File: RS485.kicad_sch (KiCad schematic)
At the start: 0 parts

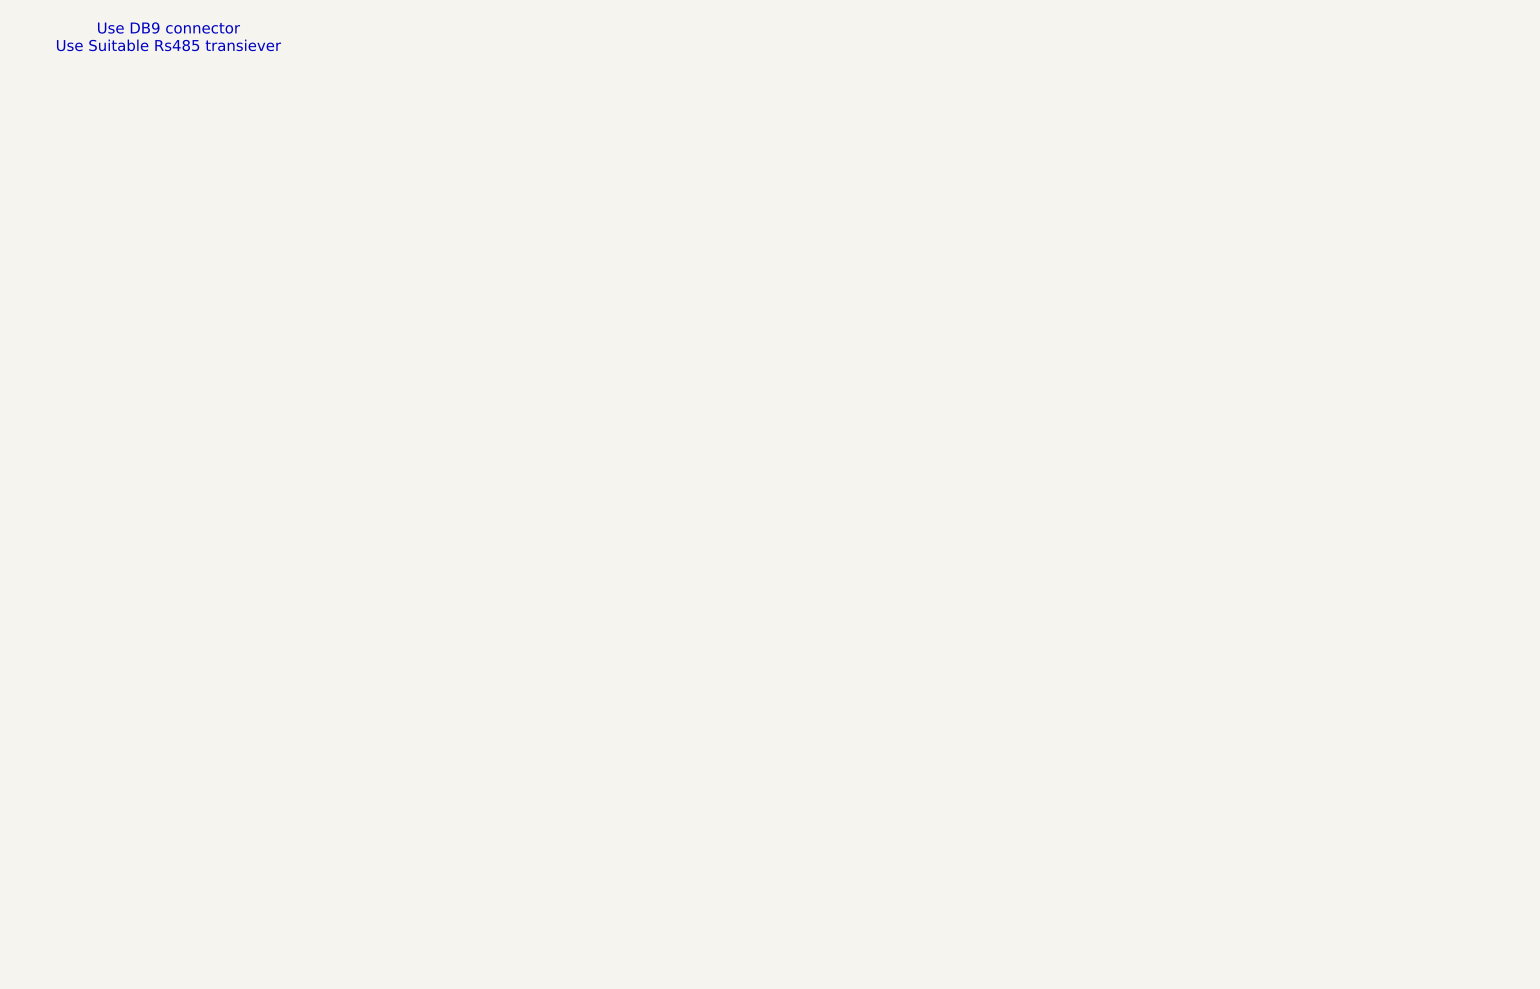
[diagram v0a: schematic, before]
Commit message: Latest updates
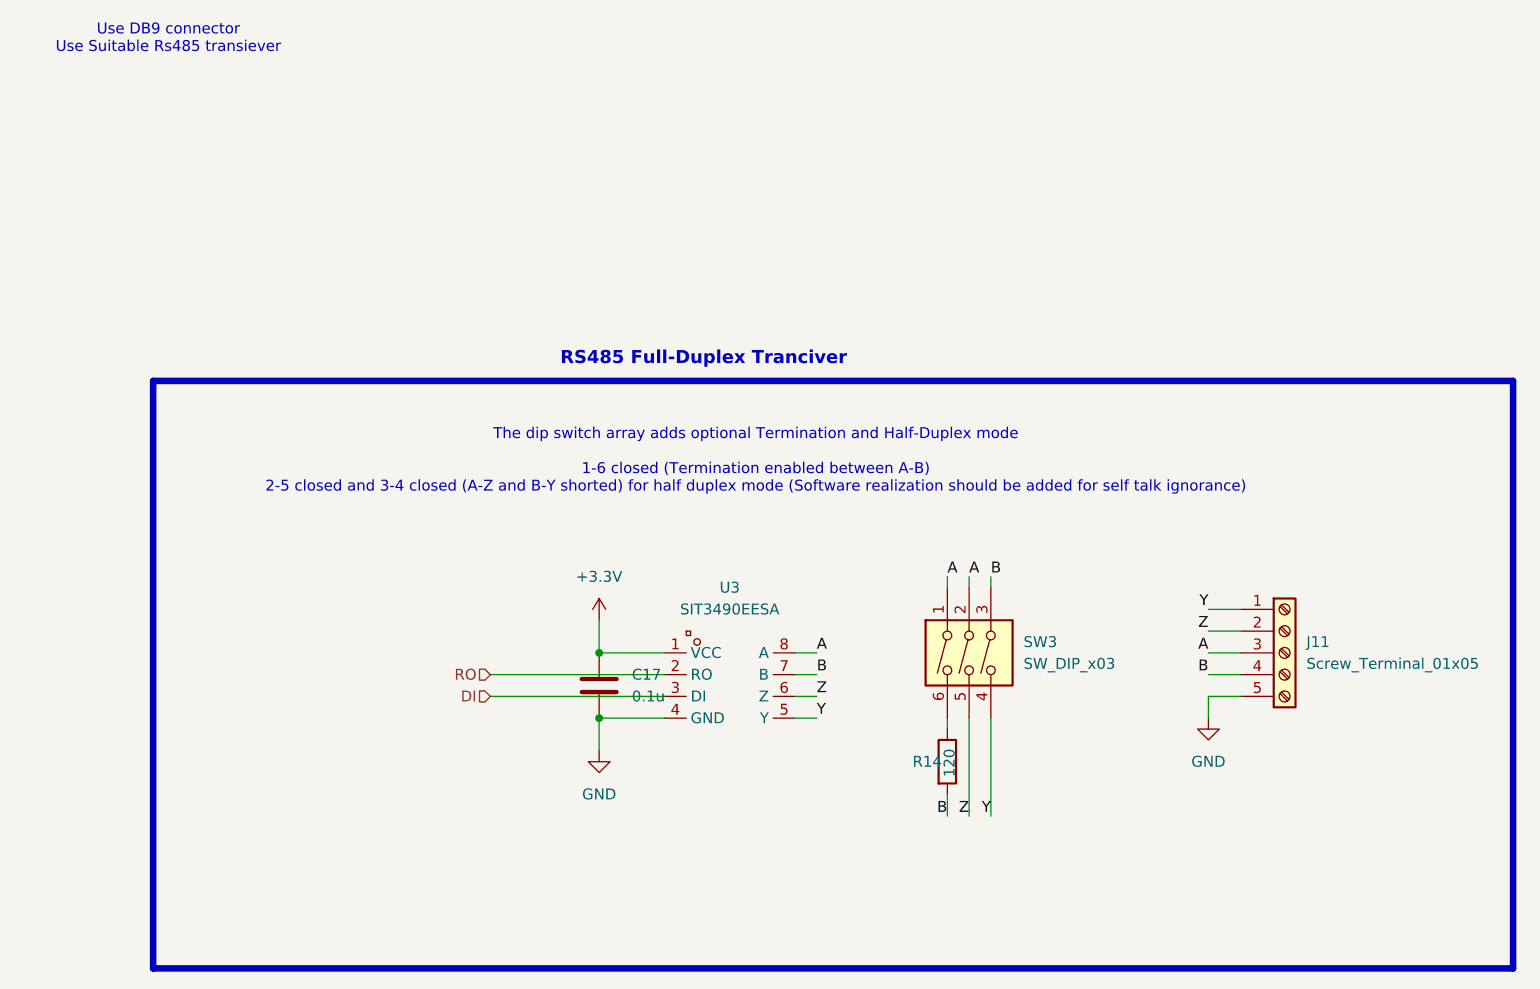
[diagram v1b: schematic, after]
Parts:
- added C17: 0.1u, symbol Device:C
- added J11: Screw_Terminal_01x05, symbol Connector:Screw_Terminal_01x05
- added R14: 120, symbol Device:R
- added SW3: SW_DIP_x03, symbol Switch:SW_DIP_x03
- added U3: SIT3490EESA, EasyEDA:SOP-8_L4.9-W3.9-P1.27-LS6.0-BL, symbol EasyEDA:SIT3490EESA
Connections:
- new net: R14.1, SW3.6
- new net +3.3V: C17.1, U3.1 (VCC)
- new net A: J11.3 (Pin_3), SW3.1, SW3.2, U3.8 (A)
- new net B: J11.4 (Pin_4), R14.2, SW3.3, U3.7 (B)
- new net DI: U3.3 (DI)
- new net GND: C17.2, J11.5 (Pin_5), U3.4 (GND)
- new net RO: U3.2 (RO)
- new net Y: J11.1 (Pin_1), SW3.4, U3.5 (Y)
- new net Z: J11.2 (Pin_2), SW3.5, U3.6 (Z)
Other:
- note added: "RS485 Full-Duplex Tranciver"
- note added: "The dip switch array adds optional Termination and Half-Duplex mode 1-6 closed (Termination enabled between A-B) 2-5 closed and 3-4 closed (A-Z and B-Y shorted) for half duplex mode (Software realization should be added for self talk ignorance)"
